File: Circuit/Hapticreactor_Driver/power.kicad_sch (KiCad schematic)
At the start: 7 parts, among them IC1 XCL103D503CR-G, J3 Conn_01x02

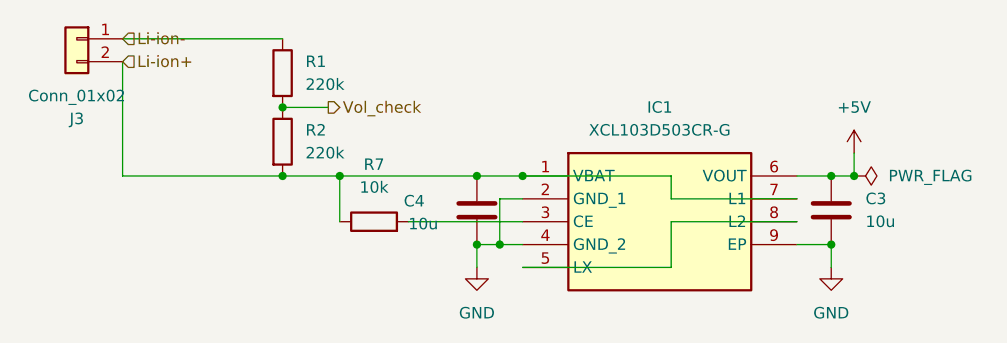
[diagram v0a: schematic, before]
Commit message: ハプティックリアクタ用基板完成
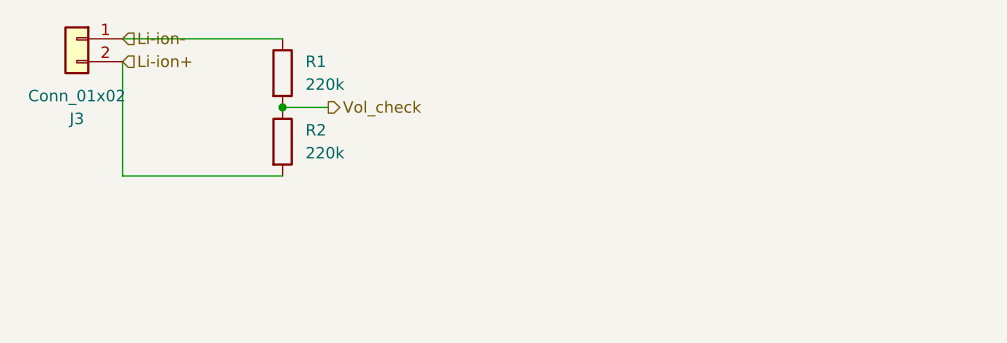
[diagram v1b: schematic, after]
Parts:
- removed C3, C4: 10u, Capacitor_SMD:C_1206_3216Metric_Pad1.33x1.80mm_HandSolder, symbol Device:C
- removed IC1: XCL103D503CR-G, XCL103D503CRG, symbol XCL103D503CR-G:XCL103D503CR-G
- removed R7: 10k, Resistor_SMD:R_0603_1608Metric_Pad0.98x0.95mm_HandSolder, symbol Device:R
